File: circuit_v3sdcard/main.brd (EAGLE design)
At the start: 46.9 x 59.4 mm, 21 parts, among them CN1 SD, CN4 5035481020, IC1 C8051F381-GM, IC3 MT29F2G01ABAGDWB, IC4 KC2016K48.0000C1GE00, IC6 MPU-9250

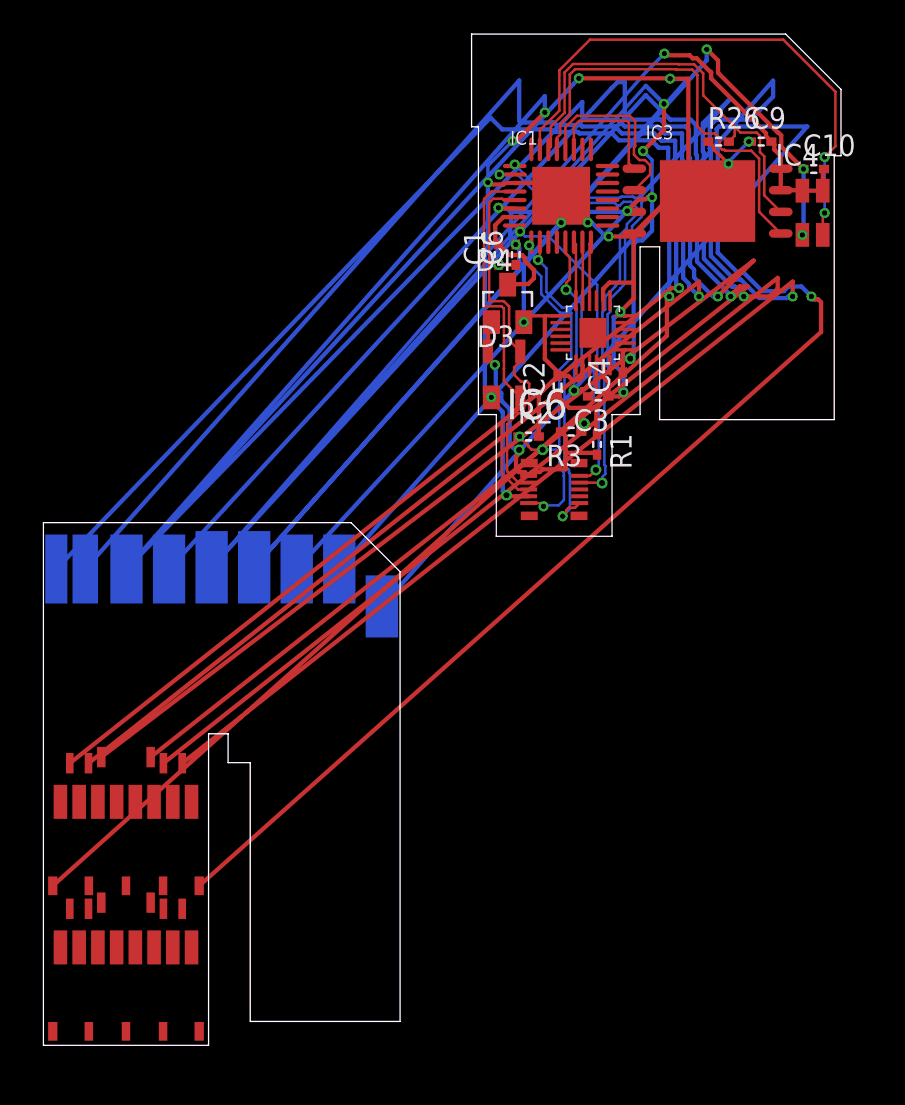
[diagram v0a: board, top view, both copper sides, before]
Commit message: Modified circuit
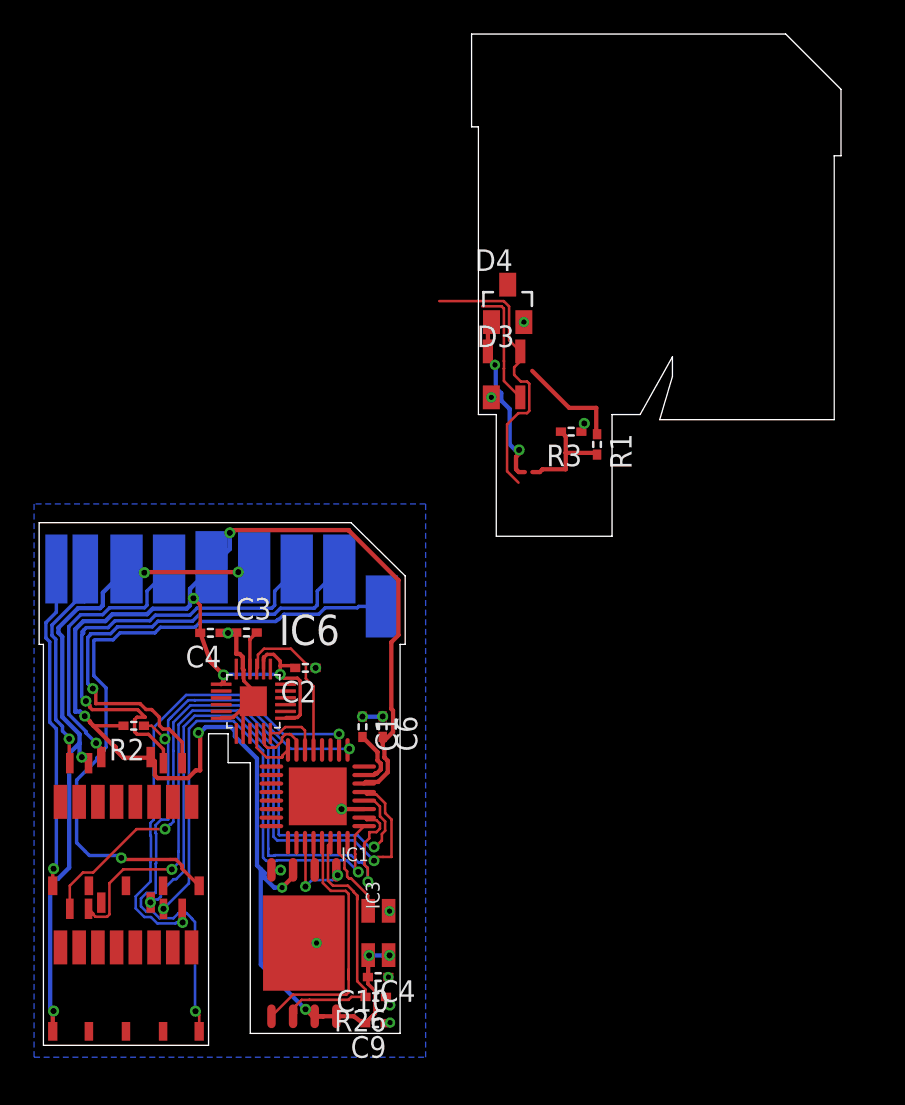
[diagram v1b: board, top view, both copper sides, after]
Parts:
- removed CN4: 5035481020, Connector:5035481020
- moved C9 56.5 mm to (19.6, 1.00), turned to 180 degrees
- moved R26 54.1 mm to (19.6, 2.54), turned to 180 degrees
- moved C10 53.9 mm to (19.7, 3.71), turned to 180 degrees
- moved IC3 49.6 mm to (15.3, 5.71), turned to 270 degrees
- moved IC4 49.4 mm to (19.7, 6.30), turned to 90 degrees
- moved IC1 38.1 mm to (16.2, 14.3), turned to 180 degrees
- moved IC6 29.4 mm to (12.4, 19.9), turned to 180 degrees
- moved C1 28.9 mm to (18.8, 18.4), turned to 270 degrees
- moved C6 28.8 mm to (20.0, 18.4), turned to 270 degrees
- moved R2 28.8 mm to (5.36, 18.5), turned to 180 degrees
- moved C4 28.3 mm to (9.86, 23.9), turned to 180 degrees
- moved C3 24.9 mm to (12.0, 23.9), turned to 0 degrees
- moved C2 22.2 mm to (15.4, 21.9), turned to 180 degrees
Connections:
- net C2CK: no longer CN4.9
- net C2D: no longer CN4.10
- net D+: no longer CN4.5
- net D-: no longer CN4.3
- net DGND: now also IC6.B; no longer CN4.7
- net RX1: no longer CN4.4
- net TX1: no longer CN4.2
- net VBUS: no longer CN4.1
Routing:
- net DGND: track 358.5 -> 61.4 mm, vias 19 -> 16
- net +3V3: track 242.3 -> 108.1 mm, vias 10 -> 11
- net N$3: track 104.6 -> 13.0 mm
- net N$6: track 107.3 -> 16.3 mm
- net N$2: track 107.5 -> 19.2 mm
- net N$12: track 103.9 -> 28.8 mm
- net N$10: track 100.0 -> 27.3 mm
- net N$14: track 108.6 -> 39.0 mm
- net D-: track 21.8 -> 57.2 mm, vias 0 -> 2
- net N$11: track 32.1 -> 4.78 mm, vias 2 -> 0
- net D+: track 22.0 -> 44.4 mm, vias 0 -> 2
- net N$4: track 15.3 -> 0.56 mm, vias 2 -> 1
- net C2CK: track 22.4 -> 37.0 mm, vias 4 -> 3
- net EEPROM_MOSI: track 25.2 -> 15.7 mm
- net EEPROM_SCK: track 25.1 -> 15.8 mm
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- added copper zone on layer 16, net DGND
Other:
- board size 46.9 x 59.4 mm -> 47.1 x 59.4 mm
